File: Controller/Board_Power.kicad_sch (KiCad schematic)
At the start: 67 parts, among them J10 Screw_Terminal_01x08, J59 USB4140-GF-0070-C_REVA3, J60 Conn_01x03_Pin, U15 LM76005RNPR, U8 LM706A0RRXR, U9 LM706A0RRXR

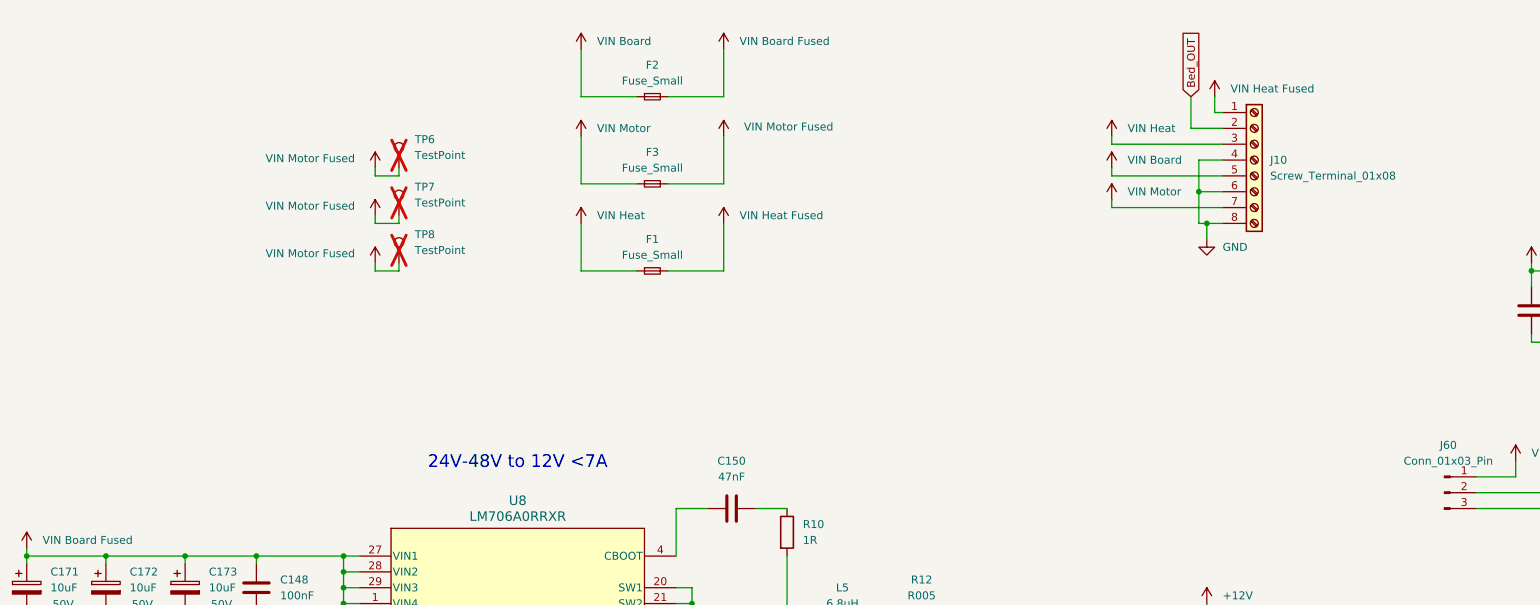
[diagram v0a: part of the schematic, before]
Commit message: REV 1B
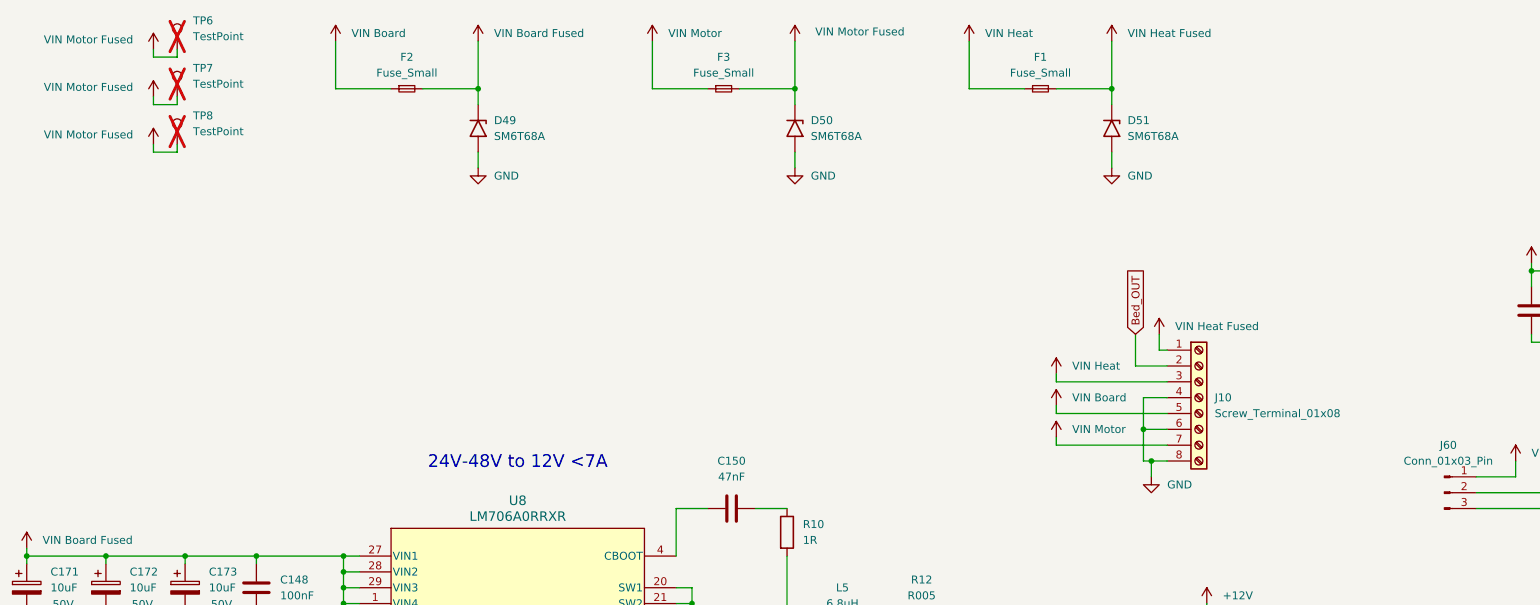
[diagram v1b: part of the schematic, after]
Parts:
- added D49, D50, D51: SM6T68A, Diode_SMD:D_SMB, symbol Diode:SM6T68A
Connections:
- net GND: now also D49.2 (A2), D50.2 (A2), D51.2 (A2)
- net VIN Board Fused: now also D49.1 (A1)
- net VIN Heat Fused: now also D51.1 (A1)
- net VIN Motor Fused: now also D50.1 (A1)
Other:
- moved on the sheet: F1, F2, F3, J10, TP6, TP7, TP8
